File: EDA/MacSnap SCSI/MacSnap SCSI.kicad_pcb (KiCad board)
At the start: 2 copper layers, 84 x 88 mm, 36 parts, among them IC1 Z53C8003VSG, IC2 MC34268DR2G, IC3 MC34268DR2G, J1 SCSI IDC-50, J2 SCSI IDC-26, U1 MB_LOW, U2 MB_HI, U3 ROM_LOW, U4 ROM_HI, U5 ATF16V8B, U6 ATF16V8B

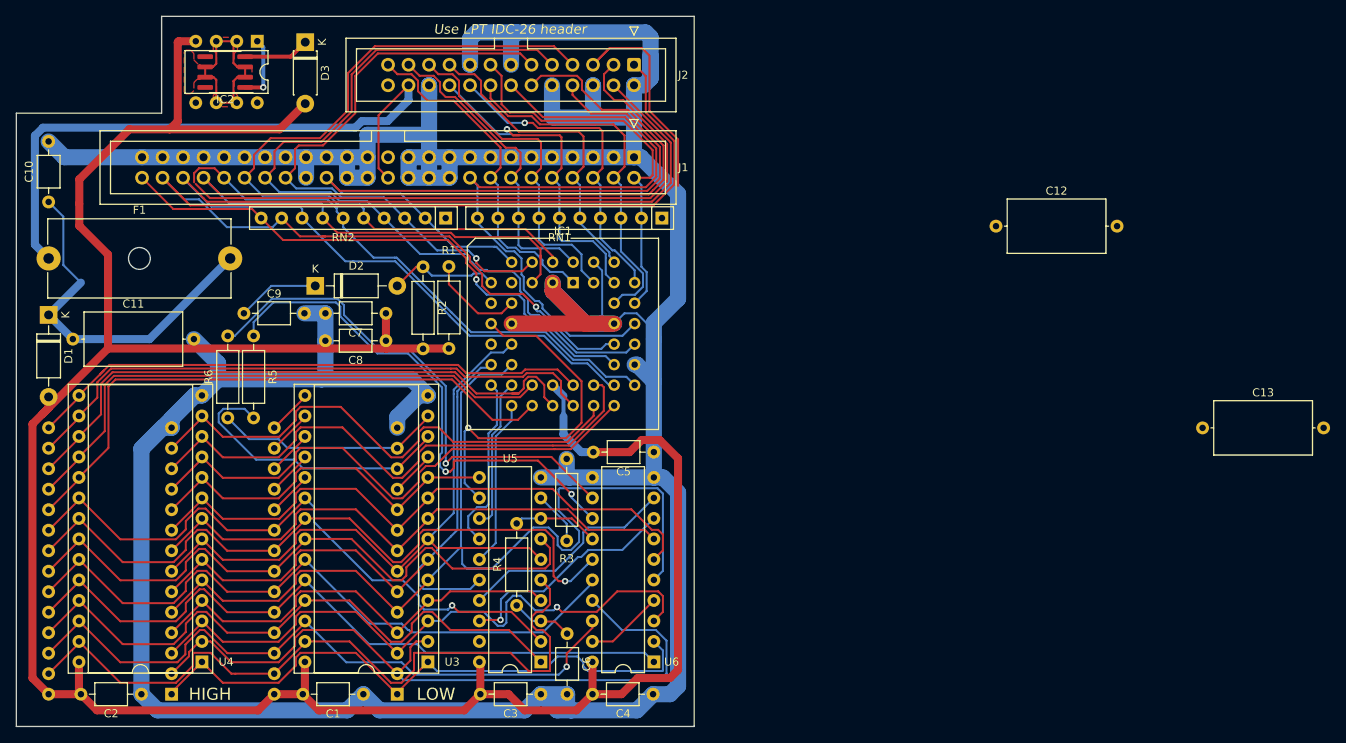
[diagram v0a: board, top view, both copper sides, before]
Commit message: MacSnap SCSI pre-2.0 cleaning
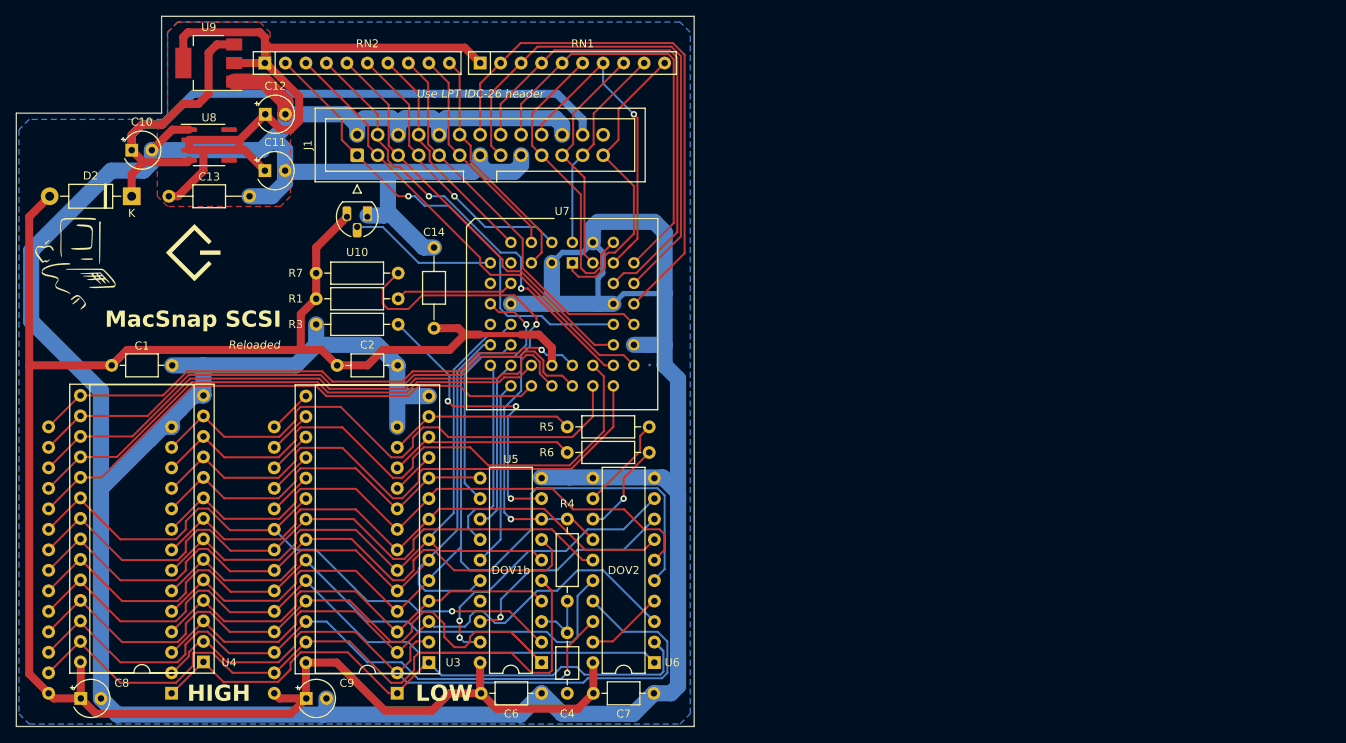
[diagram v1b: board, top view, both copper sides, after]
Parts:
- removed C3, C5: 100nF, Capacitor_THT:C_Axial_L3.8mm_D2.6mm_P7.50mm_Horizontal
- removed D1: D, Diode_THT:D_DO-41_SOD81_P10.16mm_Horizontal
- removed D3: 1N5819, Diode_THT:D_DO-41_SOD81_P7.62mm_Horizontal
- removed F1: Fuse 1.25A, Fuse:Fuseholder_Cylinder-5x20mm_Schurter_0031_8201_Horizontal_Open
- removed IC1: Z53C8003VSG, Package_LCC:PLCC-44_THT-Socket
- removed IC2: MC34268DR2G, Package_SO:SOIC-8_3.9x4.9mm_P1.27mm
- removed IC3: MC34268DR2G, Package_DIP:DIP-8_W7.62mm
- removed J2: SCSI IDC-26, Connector_IDC:IDC-Header_2x13_P2.54mm_Vertical
- removed R2: 10k, Resistor_THT:R_Axial_DIN0207_L6.3mm_D2.5mm_P10.16mm_Horizontal
- added C14: 100nF, Capacitor_THT:C_Axial_L3.8mm_D2.6mm_P10.00mm_Horizontal, F.Cu at (111.8, 90.6)
- added G***: LOGO, Misc:Macintosh logo, F.Cu at (67.3, 82.5)
- added G***: LOGO, Misc:SCSI_logo, F.Cu at (81.9, 81.3)
- added R7: 1200, Resistor_THT:R_Axial_DIN0207_L6.3mm_D2.5mm_P10.16mm_Horizontal, F.Cu at (97.2, 83.8)
- added U10: DS1233D, Package_TO_SOT_THT:TO-92_HandSolder, F.Cu at (103.5, 76.8)
- added U7: Z53C8003VSG, Package_LCC:PLCC-44_THT-Socket, F.Cu at (128.9, 82.5)
- added U8: MC34268DR2G, Package_SO:SOIC-8_3.9x4.9mm_P1.27mm, F.Cu at (83.9, 67.9)
- added U9: LT1117-2.85, Package_TO_SOT_SMD:SOT-223-3_TabPin2, F.Cu at (83.8, 57.8)
- C10: value 100nF -> 10uF; footprint Capacitor_THT:C_Axial_L3.8mm_D2.6mm_P7.50mm_Horizontal -> Capacitor_THT:CP_Radial_Tantal_D4.5mm_P2.50mm
- C11: value 2.2uF -> 10uF; footprint Capacitor_THT:C_Axial_L12.0mm_D6.5mm_P15.00mm_Horizontal -> Capacitor_THT:CP_Radial_Tantal_D4.5mm_P2.50mm
- C12: footprint Capacitor_THT:C_Axial_L12.0mm_D6.5mm_P15.00mm_Horizontal -> Capacitor_THT:CP_Radial_Tantal_D4.5mm_P2.50mm
- C13: value 10uF -> 100nF; footprint Capacitor_THT:C_Axial_L12.0mm_D6.5mm_P15.00mm_Horizontal -> Capacitor_THT:C_Axial_L3.8mm_D2.6mm_P10.00mm_Horizontal
- C4: value 100nF -> 1500pF
- C7: value C -> 100nF
- C8, C9: value C -> 10uF; footprint Capacitor_THT:C_Axial_L3.8mm_D2.6mm_P7.50mm_Horizontal -> Capacitor_THT:CP_Radial_Tantal_D4.5mm_P2.50mm
- D2: value 1N4001 -> 1N5817
- J1: value SCSI IDC-50 -> SCSI IDC-26; footprint Connector_IDC:IDC-Header_2x25_P2.54mm_Vertical -> Connector_IDC:IDC-Header_2x13_P2.54mm_Vertical
- moved C13 131.3 mm to (78.9, 74.3)
- moved C12 91.6 mm to (90.8, 64.1)
- moved C8 58.3 mm to (68.0, 136.5), turned to 0 degrees
- moved C7 53.6 mm to (131.5, 135.9), turned to 0 degrees
- moved R6 52.4 mm to (138.4, 106.0), turned to 180 degrees
- moved C2 51.7 mm to (99.8, 95.2)
- moved C1 51.3 mm to (71.8, 95.2), turned to 0 degrees
- moved C9 48.3 mm to (95.9, 136.5)
- moved R5 40.5 mm to (128.3, 102.9), turned to 0 degrees
- moved J1 34.3 mm to (102.2, 69.2), turned to 90 degrees
- moved R3 34.0 mm to (107.3, 90.2), turned to 180 degrees
- moved C11 31.7 mm to (90.8, 71.1)
- moved RN1 29.6 mm to (117.5, 57.8), turned to 0 degrees
- moved RN2 29.5 mm to (90.8, 57.8), turned to 0 degrees
- moved D2 25.3 mm to (74.3, 74.3), turned to 180 degrees
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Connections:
- net /A17 renamed /~{ROM}
- net /~ROMCE renamed /A20
- C1 pad 1: GND -> VCC
- C1 pad 2: VCC -> GND
- C10 pad 1: Net-(C10-Pad1) -> TMPWR
- C11 pad 1: Net-(C10-Pad1) -> +2V8
- C12 pad 1: Net-(C12-Pad1) -> +2V8
- C4 pad 1: VCC -> Net-(U5-I3)
- C6 pad 1: Net-(C6-Pad1) -> VCC
- C9 pad 1: Net-(C9-Pad1) -> VCC
- D2 pad 1: Net-(C9-Pad1) -> TMPWR
- D2 pad 2: Net-(D2-Pad2) -> VCC
- J1 pad 1: GND -> /~{REQ}
- J1 pad 10: /DB4 -> GND
- J1 pad 11: GND -> /~{BSY}
- J1 pad 12: /DB5 -> /~{SEL}
- J1 pad 14: /DB6 -> /PARITY
- J1 pad 15: GND -> /DB0
- J1 pad 16: /DB7 -> /DB1
- J1 pad 18: /PARITY -> /DB2
- J1 pad 19: GND -> /DB3
- J1 pad 2: /DB0 -> GND
- J1 pad 20: GND -> /DB4
- J1 pad 21: GND -> /DB5
- J1 pad 23: GND -> /DB6
- J1 pad 24: GND -> TMPWR
- J1 pad 25: (no net) -> /DB7
- J1 pad 26: TMPWR -> unconnected-(J1-Pin_26-Pad26)
- J1 pad 3: GND -> /~{MSG}
- J1 pad 4: /DB1 -> /~{CD}
- J1 pad 5: GND -> /~{IO}
- J1 pad 6: /DB2 -> GND
- J1 pad 7: GND -> /~{RST}
- J1 pad 8: /DB3 -> /~{ATN}
- J1 pad 9: GND -> /~{ACK}
- R4 pad 1: Net-(C6-Pad1) -> Net-(U5-I3)
- R5 pad 1: Net-(R5-Pad1) -> /D2
- R5 pad 2: /D1 -> Net-(U6-IO8)
- R6 pad 1: /D2 -> Net-(U6-IO7)
- R6 pad 2: Net-(R6-Pad2) -> /D1
- RN1 pad 10: /PARITY -> /DB7
- RN1 pad 2: /DB0 -> /PARITY
- RN1 pad 3: /DB1 -> /DB0
- RN1 pad 4: /DB2 -> /DB1
- RN1 pad 5: /DB3 -> /DB2
- RN1 pad 6: /DB4 -> /DB3
- RN1 pad 7: /DB5 -> /DB4
- RN1 pad 8: /DB6 -> /DB5
- RN1 pad 9: /DB7 -> /DB6
- RN2 pad 10: /~IO -> /~{SEL}
- RN2 pad 2: /~ATN -> /~{REQ}
- RN2 pad 3: /~BSY -> /~{MSG}
- RN2 pad 4: /~ACK -> /~{CD}
- RN2 pad 5: /~RST -> /~{IO}
- RN2 pad 6: /~MSG -> /~{RST}
- RN2 pad 7: /~SEL -> /~{ATN}
- RN2 pad 8: /~CD -> /~{ACK}
- RN2 pad 9: /~REQ -> /~{BSY}
- U5 pad 12: /~DACK -> /~{DACK}
- U5 pad 13: /~IOR -> /~{IOR}
- U5 pad 14: /~CS -> /~{CS}
- U5 pad 15: /~IOW -> /~{IOW}
- U5 pad 17: Net-(U5-Pad17) -> unconnected-(U5-I03-Pad17)
- U5 pad 19: (no net) -> Net-(U5-IO1)
- U5 pad 3: Net-(C6-Pad1) -> Net-(U5-I3)
- U6 pad 12: Net-(R6-Pad2) -> Net-(U6-IO8)
- U6 pad 13: Net-(R5-Pad1) -> Net-(U6-IO7)
- U6 pad 9: Net-(U5-Pad17) -> Net-(U5-IO1)
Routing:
- net /~REQ: track 155.3 -> 0.00 mm, vias 1 -> 0
- net /~MSG: track 147.2 -> 0.00 mm
- net /~CD: track 142.5 -> 0.00 mm
- net /~SEL: track 135.2 -> 0.00 mm
- net /~ACK: track 104.4 -> 0.00 mm
- net /~IO: track 99.0 -> 0.00 mm, vias 1 -> 0
- net /~RST: track 95.6 -> 0.00 mm
- net /~ATN: track 88.5 -> 0.00 mm
- net /~BSY: track 77.6 -> 0.00 mm, vias 1 -> 0
- net +2V8: track 25.3 -> 94.5 mm
- net Net-(R5-Pad1): track 64.4 -> 0.00 mm, vias 2 -> 0
- net Net-(R6-Pad2): track 64.3 -> 0.00 mm, vias 1 -> 0
- net VCC: track 315.9 -> 252.3 mm
- net /~{REQ}: track 0.00 -> 59.3 mm, vias 0 -> 1
- net /~{MSG}: track 0.00 -> 58.1 mm
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- added copper zone on B.Cu, net GND
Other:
- net class Default removed
- net class GND removed
- net class VCC removed
- board text added: "DOV1b"
- board text added: "DOV2"
- board text added: "JLCJLCJLC"
- board text added: "MacSnap SCSI"
- board text added: "MacSnap SCSI Reloaded © 2023 Michel Depeige Based on DOVE MacSnap SCSI https://github.com/demik/oldworld"
- board text added: "Reloaded"
